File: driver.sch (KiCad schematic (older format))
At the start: 48 parts, among them J1 Screw_Terminal_01x02, J2 Conn_02x16_Odd_Even, Q1 Q_NMOS_GDSD, Q10 Q_NMOS_GDSD, Q11 Q_NMOS_GDSD, Q12 Q_NMOS_GDSD, Q13 Q_NMOS_GDSD, Q14 Q_NMOS_GDSD, Q15 Q_NMOS_GDSD, Q16 Q_NMOS_GDSD, Q17 AOD417 Q_PMOS_DGS, Q2 Q_NMOS_GDSD, Q3 Q_NMOS_GDSD, Q4 Q_NMOS_GDSD, Q5 Q_NMOS_GDSD, Q6 Q_NMOS_GDSD, Q7 Q_NMOS_GDSD, Q8 Q_NMOS_GDSD, Q9 Q_NMOS_GDSD, SW1 SW_Push, U1 PCA9685PW

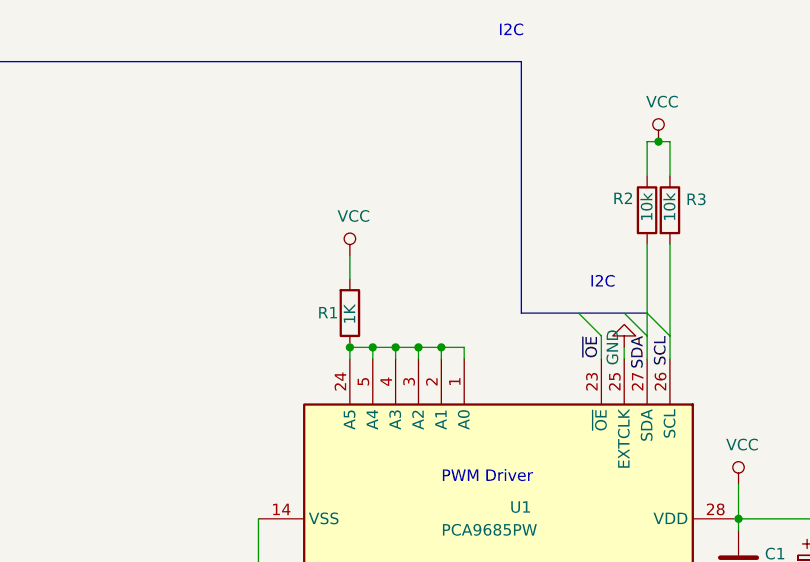
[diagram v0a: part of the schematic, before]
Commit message: change address
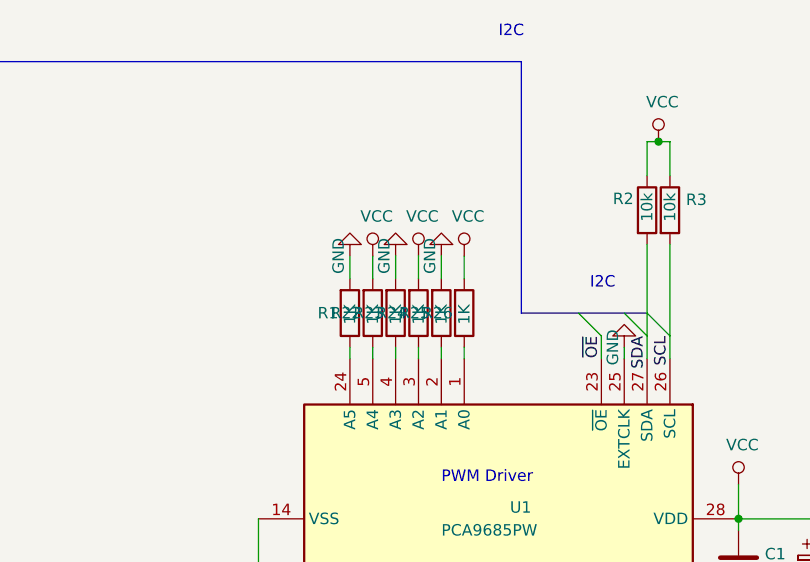
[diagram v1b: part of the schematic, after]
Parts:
- added R22, R23, R24, R25, R26: 1K, Resistor_SMD:R_0805_2012Metric_Pad1.15x1.40mm_HandSolder, symbol Device:R
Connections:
- net GND: now also R1.2, R23.2, R25.2
- net VCC: now also R22.2, R24.2, R26.2; no longer R1.2
- new net: R26.1, U1.1 (A0)
- new net: R25.1, U1.2 (A1)
- new net: R1.1, U1.24 (A5)
- new net: R24.1, U1.3 (A2)
- new net: R23.1, U1.4 (A3)
- new net: R22.1, U1.5 (A4)
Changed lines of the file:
@@
 L power:VCC #PWR0107
 U 1 1 5C1B585A
-P 5100 1900
-F 0 "#PWR0107" H 5100 1750 50  0001 C CNN
-F 1 "VCC" H 5117 2073 50  0000 C CNN
-F 2 "" H 5100 1900 50  0001 C CNN
-F 3 "" H 5100 1900 50  0001 C CNN
-	1    5100 1900
+P 5200 1900
+F 0 "#PWR0107" H 5200 1750 50  0001 C CNN
+F 1 "VCC" H 5217 2073 50  0000 C CNN
+F 2 "" H 5200 1900 50  0001 C CNN
+F 3 "" H 5200 1900 50  0001 C CNN
+	1    5200 1900
 	1    0    0    -1
 $EndComp
 Wire Wire Line
 	5100 2300 5100 2350
-Wire Wire Line
-	5200 2300 5200 2350
-Wire Wire Line
-	5300 2300 5300 2350
-Wire Wire Line
-	5400 2300 5400 2350
-Wire Wire Line
-	5500 2300 5500 2350
-Wire Wire Line
-	5600 2300 5600 2350
-Wire Wire Line
-	5100 1900 5100 2000
 $Comp
 L Device:R R1
@@
 Text Notes 10500 1700 0    157  ~ 0
 change footprint of big caps
-Wire Wire Line
-	5100 2300 5200 2300
-Connection ~ 5100 2300
-Wire Wire Line
-	5200 2300 5300 2300
-Connection ~ 5200 2300
-Connection ~ 5300 2300
-Wire Wire Line
-	5300 2300 5400 2300
-Connection ~ 5400 2300
-Wire Wire Line
-	5400 2300 5500 2300
-Wire Wire Line
-	5600 2300 5500 2300
-Connection ~ 5500 2300
 $Comp
 L Device:R_Small R4
@@
 	6500 1850 6500 2350
 $Comp
-L power:GND #PWR?
+L power:GND #PWR0106
 U 1 1 5C4D7BC3
 P 6300 2300
-F 0 "#PWR?" H 6300 2050 50  0001 C CNN
+F 0 "#PWR0106" H 6300 2050 50  0001 C CNN
 F 1 "GND" V 6350 2300 50  0000 C CNN
 F 2 "" H 6300 2300 50  0001 C CNN
@@
 Wire Wire Line
 	6300 2300 6300 2350
+$Comp
+L Device:R R23
+U 1 1 5C4E9154
+P 5300 2150
+F 0 "R23" H 5250 2150 50  0000 R CNN
+F 1 "1K" V 5300 2200 50  0000 R CNN
+F 2 "Resistor_SMD:R_0805_2012Metric_Pad1.15x1.40mm_HandSolder" V 5230 2150 50  0001 C CNN
+F 3 "~" H 5300 2150 50  0001 C CNN
+	1    5300 2150
+	1    0    0    1
+$EndComp
+$Comp
+L Device:R R24
+U 1 1 5C4E91D2
+P 5400 2150
+F 0 "R24" H 5350 2150 50  0000 R CNN
+F 1 "1K" V 5400 2200 50  0000 R CNN
+F 2 "Resistor_SMD:R_0805_2012Metric_Pad1.15x1.40mm_HandSolder" V 5330 2150 50  0001 C CNN
+F 3 "~" H 5400 2150 50  0001 C CNN
+	1    5400 2150
+	1    0    0    1
+$EndComp
+$Comp
+L Device:R R22
+U 1 1 5C4E92AE
+P 5200 2150
+F 0 "R22" H 5150 2150 50  0000 R CNN
+F 1 "1K" V 5200 2200 50  0000 R CNN
+F 2 "Resistor_SMD:R_0805_2012Metric_Pad1.15x1.40mm_HandSolder" V 5130 2150 50  0001 C CNN
+F 3 "~" H 5200 2150 50  0001 C CNN
+	1    5200 2150
+	1    0    0    1
+$EndComp
+$Comp
+L Device:R R25
+U 1 1 5C4E9324
+P 5500 2150
+F 0 "R25" H 5450 2150 50  0000 R CNN
+F 1 "1K" V 5500 2200 50  0000 R CNN
+F 2 "Resistor_SMD:R_0805_2012Metric_Pad1.15x1.40mm_HandSolder" V 5430 2150 50  0001 C CNN
+F 3 "~" H 5500 2150 50  0001 C CNN
+	1    5500 2150
+	1    0    0    1
+$EndComp
+$Comp
+L Device:R R26
+U 1 1 5C4E939C
+P 5600 2150
+F 0 "R26" H 5550 2150 50  0000 R CNN
+F 1 "1K" V 5600 2200 50  0000 R CNN
+F 2 "Resistor_SMD:R_0805_2012Metric_Pad1.15x1.40mm_HandSolder" V 5530 2150 50  0001 C CNN
+F 3 "~" H 5600 2150 50  0001 C CNN
+	1    5600 2150
+	1    0    0    1
+$EndComp
+$Comp
+L power:VCC #PWR0109
+U 1 1 5C4E94F8
+P 5400 1900
+F 0 "#PWR0109" H 5400 1750 50  0001 C CNN
+F 1 "VCC" H 5417 2073 50  0000 C CNN
+F 2 "" H 5400 1900 50  0001 C CNN
+F 3 "" H 5400 1900 50  0001 C CNN
+	1    5400 1900
+	1    0    0    -1
+$EndComp
+$Comp
+L power:VCC #PWR0110
+U 1 1 5C4E956D
+P 5600 1900
+F 0 "#PWR0110" H 5600 1750 50  0001 C CNN
+F 1 "VCC" H 5617 2073 50  0000 C CNN
+F 2 "" H 5600 1900 50  0001 C CNN
+F 3 "" H 5600 1900 50  0001 C CNN
+	1    5600 1900
+	1    0    0    -1
+$EndComp
+$Comp
+L power:GND #PWR0111
+U 1 1 5C4E95E2
+P 5100 1900
+F 0 "#PWR0111" H 5100 1650 50  0001 C CNN
+F 1 "GND" V 5150 1900 50  0000 C CNN
+F 2 "" H 5100 1900 50  0001 C CNN
+F 3 "" H 5100 1900 50  0001 C CNN
+	1    5100 1900
+	-1   0    0    1
+$EndComp
+$Comp
+L power:GND #PWR0112
+U 1 1 5C4E9657
+P 5300 1900
+F 0 "#PWR0112" H 5300 1650 50  0001 C CNN
+F 1 "GND" V 5350 1900 50  0000 C CNN
+F 2 "" H 5300 1900 50  0001 C CNN
+F 3 "" H 5300 1900 50  0001 C CNN
+	1    5300 1900
+	-1   0    0    1
+$EndComp
+$Comp
+L power:GND #PWR0113
+U 1 1 5C4E96CC
+P 5500 1900
+F 0 "#PWR0113" H 5500 1650 50  0001 C CNN
+F 1 "GND" V 5550 1900 50  0000 C CNN
+F 2 "" H 5500 1900 50  0001 C CNN
+F 3 "" H 5500 1900 50  0001 C CNN
+	1    5500 1900
+	-1   0    0    1
+$EndComp
+Wire Wire Line
+	5100 1900 5100 2000
+Wire Wire Line
+	5200 1900 5200 2000
+Wire Wire Line
+	5300 1900 5300 2000
+Wire Wire Line
+	5400 1900 5400 2000
+Wire Wire Line
+	5500 1900 5500 2000
+Wire Wire Line
+	5600 1900 5600 2000
+Wire Wire Line
+	5200 2300 5200 2350
+Wire Wire Line
+	5300 2300 5300 2350
+Wire Wire Line
+	5400 2300 5400 2350
+Wire Wire Line
+	5500 2300 5500 2350
+Wire Wire Line
+	5600 2300 5600 2350
 Wire Wire Line
 	6400 1850 6400 2350
